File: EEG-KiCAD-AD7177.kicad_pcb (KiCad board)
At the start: 2 copper layers, 35.6 x 21.7 mm, 53 parts, among them J1 IN EEG, J2 Battery, J3 Programmer, J4 Vs+ Ele, J5 Vs- Ele, U1 AD7177-2, U2 OPA2210, U3 NRF528XX-QFAA, U4 RP511Z331_3.3V, U5 XCL101A501-5V, X1 Crystal_GND24, X2 32.768 kHz, X3 FA-20H 9pF 10ppm

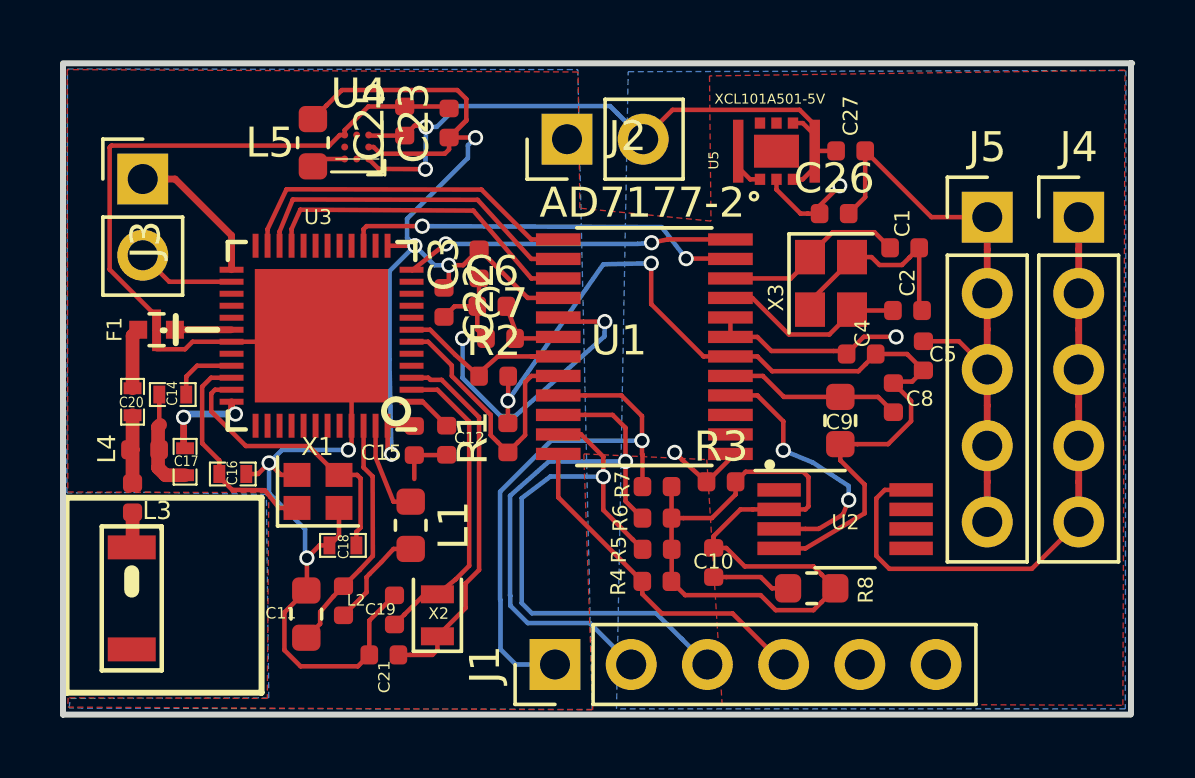
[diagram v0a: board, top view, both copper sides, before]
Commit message: With description
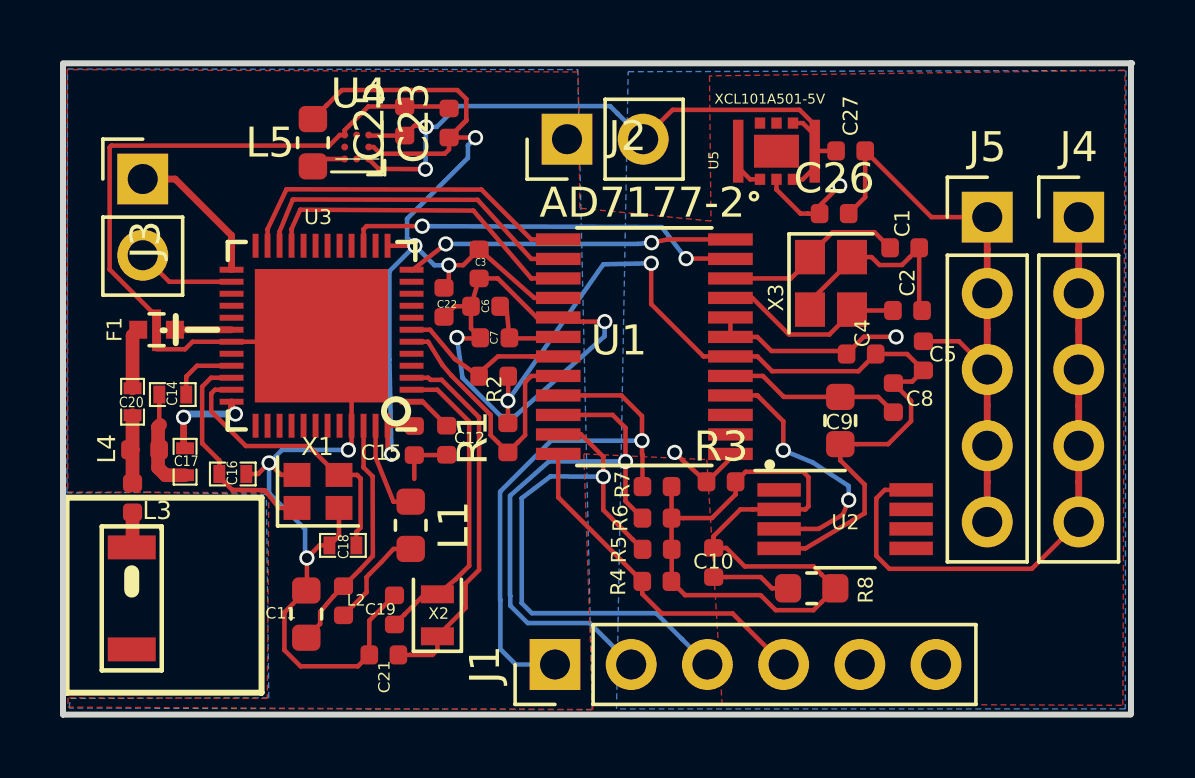
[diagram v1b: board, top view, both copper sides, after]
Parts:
- moved C6 0.21 mm to (201.2, 127.9)
- moved C7 0.19 mm to (201.5, 129.0)
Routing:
- net AGND: track 110.5 -> 113.5 mm
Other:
- board text added: "BIAS"
- board text added: "Batt+"
- board text added: "Batt-"
- board text added: "CLK"
- board text added: "IN0"
- board text added: "IN1"
- board text added: "IN2"
- board text added: "IN3"
- board text added: "IN4"
- board text added: "IO"
- board text added: "V+"
- board text added: "V-"
